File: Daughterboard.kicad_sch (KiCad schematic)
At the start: 61 parts, among them U1 SI8271GB-IS, U2 SI8271GB-IS, U3 GS61004B, U4 IES0105S09, U5 GS61004B, U6 IES0105S09

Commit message: initial version for commenting
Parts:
- TP13, TP14, TP15, TP16, TP17, TP18, TP19: footprint TestPoint:TestPoint_Pad_D2.0mm -> TestPoint:TestPoint_THTPad_D1.0mm_Drill0.5mm
- U3, U5: footprint GS61004B:GS61004B -> GS61004B:GS6XXX4B
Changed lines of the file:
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@@
 			)
 		)
-		(property "Footprint" "TestPoint:TestPoint_Pad_D2.0mm"
+		(property "Footprint" "TestPoint:TestPoint_THTPad_D1.0mm_Drill0.5mm"
 			(at 341.63 125.73 0)
 			(effects
@@
 			)
 		)
-		(property "Footprint" "TestPoint:TestPoint_Pad_D2.0mm"
+		(property "Footprint" "TestPoint:TestPoint_THTPad_D1.0mm_Drill0.5mm"
 			(at 341.503 107.823 0)
 			(effects
@@
 			)
 		)
-		(property "Footprint" "GS61004B:GS61004B"
+		(property "Footprint" "GS61004B:GS6XXX4B"
 			(at 232.41 231.14 0)
 			(effects
@@
 			)
 		)
-		(property "Footprint" "TestPoint:TestPoint_Pad_D2.0mm"
+		(property "Footprint" "TestPoint:TestPoint_THTPad_D1.0mm_Drill0.5mm"
 			(at 355.6 125.73 0)
 			(effects
@@
 			)
 		)
-		(property "Footprint" "TestPoint:TestPoint_Pad_D2.0mm"
+		(property "Footprint" "TestPoint:TestPoint_THTPad_D1.0mm_Drill0.5mm"
 			(at 325.12 125.73 0)
 			(effects
@@
 			)
 		)
-		(property "Footprint" "TestPoint:TestPoint_Pad_D2.0mm"
+		(property "Footprint" "TestPoint:TestPoint_THTPad_D1.0mm_Drill0.5mm"
 			(at 324.993 107.823 0)
 			(effects
@@
 			)
 		)
-		(property "Footprint" "TestPoint:TestPoint_Pad_D2.0mm"
+		(property "Footprint" "TestPoint:TestPoint_THTPad_D1.0mm_Drill0.5mm"
 			(at 314.96 125.73 0)
 			(effects
@@
 			)
 		)
-		(property "Footprint" "TestPoint:TestPoint_Pad_D2.0mm"
+		(property "Footprint" "TestPoint:TestPoint_THTPad_D1.0mm_Drill0.5mm"
 			(at 355.473 107.823 0)
 			(effects
@@
 			)
 		)
-		(property "Footprint" "GS61004B:GS61004B"
+		(property "Footprint" "GS61004B:GS6XXX4B"
 			(at 232.41 93.98 0)
 			(effects

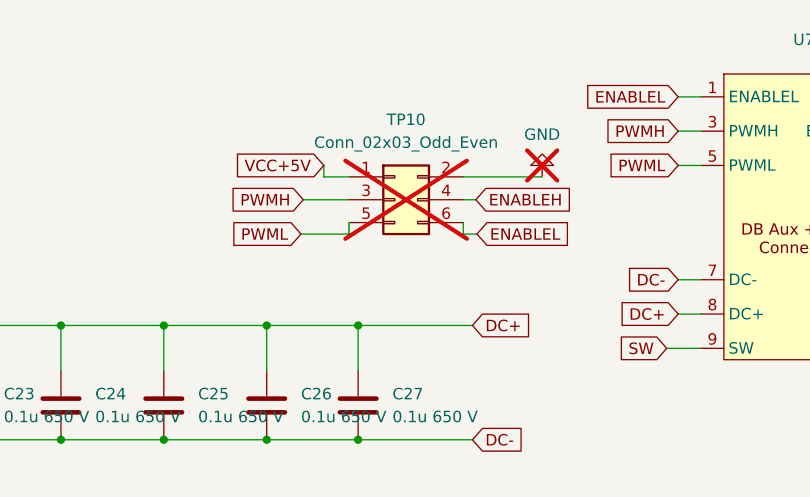
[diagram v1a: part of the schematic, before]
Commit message: fixed after comments
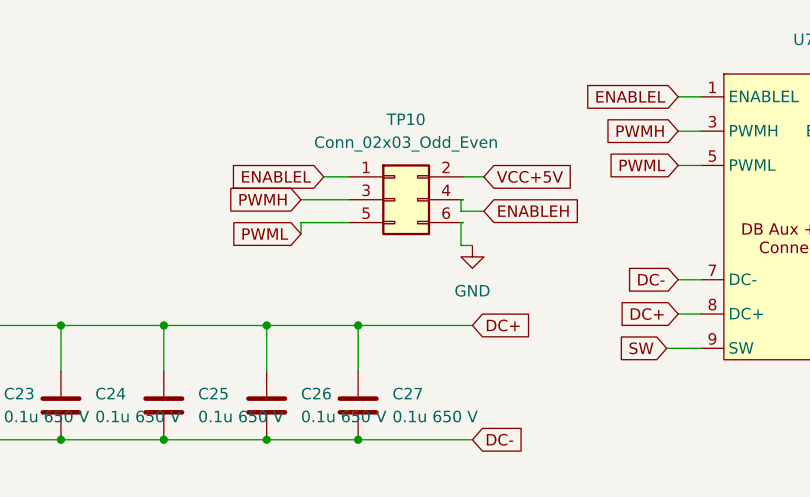
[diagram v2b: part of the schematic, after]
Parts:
- TP10: footprint (none) -> 3x2_connector:CON6_2X3_TU_TSW_SAI; now fitted
- U1, U2: footprint Package_SO:SOIC-8-1EP_3.9x4.9mm_P1.27mm_EP2.29x3mm -> Package_SO:SOIC-8_3.9x4.9mm_P1.27mm
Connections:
- net ENABLEL: now also TP10.1 (Pin_1); no longer TP10.6 (Pin_6)
- net GND: now also TP10.6 (Pin_6); no longer TP10.2 (Pin_2)
- net VCC+5V: now also TP10.2 (Pin_2); no longer TP10.1 (Pin_1)
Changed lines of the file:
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@@
 	(wire
 		(pts
-			(xy 124.46 106.68) (xy 105.41 106.68)
+			(xy 339.09 36.83) (xy 340.36 36.83)
 		)
 		(stroke
@@
 	(wire
 		(pts
-			(xy 323.85 27.94) (xy 323.85 29.21)
+			(xy 124.46 106.68) (xy 105.41 106.68)
 		)
 		(stroke
@@
 	(wire
 		(pts
+			(xy 321.31 34.29) (xy 321.31 35.56)
+		)
+		(stroke
+			(width 0)
+			(type default)
+		)
+	)
+	(wire
+		(pts
 			(xy 124.46 101.6) (xy 124.46 100.33)
 		)
@@
 	(wire
 		(pts
+			(xy 326.644 29.21) (xy 323.85 29.21)
+		)
+		(stroke
+			(width 0)
+			(type default)
+		)
+	)
+	(wire
+		(pts
 			(xy 273.05 45.72) (xy 273.05 50.8)
 		)
@@
 	(wire
 		(pts
-			(xy 339.344 35.56) (xy 339.344 34.29)
+			(xy 339.09 33.02) (xy 341.63 33.02)
 		)
 		(stroke
@@
 	(wire
 		(pts
+			(xy 339.09 34.29) (xy 339.344 34.29)
+		)
+		(stroke
+			(width 0)
+			(type default)
+		)
+	)
+	(wire
+		(pts
 			(xy 220.98 246.38) (xy 240.03 246.38)
 		)
@@
 	(wire
 		(pts
-			(xy 348.107 29.21) (xy 339.344 29.21)
-		)
-		(stroke
-			(width 0)
-			(type default)
-		)
-	)
-	(wire
-		(pts
 			(xy 176.53 24.13) (xy 176.53 26.67)
 		)
@@
 	(wire
 		(pts
+			(xy 339.09 33.02) (xy 339.09 31.75)
+		)
+		(stroke
+			(width 0)
+			(type default)
+		)
+	)
+	(wire
+		(pts
 			(xy 158.75 240.03) (xy 158.75 237.49)
 		)
@@
 	(wire
 		(pts
-			(xy 323.85 29.21) (xy 326.644 29.21)
-		)
-		(stroke
-			(width 0)
-			(type default)
-		)
-	)
-	(wire
-		(pts
 			(xy 391.16 24.13) (xy 388.62 24.13)
 		)
@@
 	(wire
 		(pts
-			(xy 326.644 35.56) (xy 326.644 34.29)
-		)
-		(stroke
-			(width 0)
-			(type default)
-		)
-	)
-	(wire
-		(pts
 			(xy 319.913 107.823) (xy 319.913 110.363)
 		)
@@
 	(wire
 		(pts
+			(xy 339.09 36.83) (xy 339.09 34.29)
+		)
+		(stroke
+			(width 0)
+			(type default)
+		)
+	)
+	(wire
+		(pts
 			(xy 190.5 185.42) (xy 179.07 185.42)
 		)
@@
 	(wire
 		(pts
-			(xy 321.564 31.75) (xy 326.644 31.75)
+			(xy 321.31 31.75) (xy 326.644 31.75)
 		)
 		(stroke
@@
 	(wire
 		(pts
+			(xy 339.09 31.75) (xy 339.344 31.75)
+		)
+		(stroke
+			(width 0)
+			(type default)
+		)
+	)
+	(wire
+		(pts
 			(xy 48.26 26.67) (xy 48.26 27.94)
 		)
@@
 	(wire
 		(pts
+			(xy 326.644 34.29) (xy 321.31 34.29)
+		)
+		(stroke
+			(width 0)
+			(type default)
+		)
+	)
+	(wire
+		(pts
 			(xy 82.55 238.76) (xy 124.46 238.76)
 		)
@@
 	(wire
 		(pts
-			(xy 340.868 35.56) (xy 339.344 35.56)
-		)
-		(stroke
-			(width 0)
-			(type default)
-		)
-	)
-	(wire
-		(pts
 			(xy 205.74 46.99) (xy 205.74 49.53)
 		)
@@
 	(wire
 		(pts
-			(xy 294.64 58.42) (xy 306.07 58.42)
+			(xy 339.344 29.21) (xy 341.63 29.21)
 		)
 		(stroke
@@
 	(wire
 		(pts
-			(xy 327.66 45.72) (xy 327.66 50.8)
+			(xy 294.64 58.42) (xy 306.07 58.42)
 		)
 		(stroke
@@
 	(wire
 		(pts
-			(xy 363.22 24.13) (xy 365.76 24.13)
+			(xy 327.66 45.72) (xy 327.66 50.8)
 		)
 		(stroke
@@
 	(wire
 		(pts
-			(xy 186.69 203.2) (xy 186.69 207.01)
+			(xy 363.22 24.13) (xy 365.76 24.13)
 		)
 		(stroke
@@
 	(wire
 		(pts
-			(xy 176.53 34.29) (xy 176.53 49.53)
+			(xy 186.69 203.2) (xy 186.69 207.01)
 		)
 		(stroke
@@
 	(wire
 		(pts
-			(xy 273.05 45.72) (xy 284.48 45.72)
+			(xy 176.53 34.29) (xy 176.53 49.53)
 		)
 		(stroke
@@
 	(wire
 		(pts
-			(xy 321.31 35.56) (xy 326.644 35.56)
+			(xy 273.05 45.72) (xy 284.48 45.72)
 		)
 		(stroke
@@
 	(wire
 		(pts
-			(xy 339.344 31.75) (xy 340.741 31.75)
-		)
-		(stroke
-			(width 0)
-			(type default)
-		)
-	)
-	(wire
-		(pts
 			(xy 82.55 101.6) (xy 124.46 101.6)
 		)
@@
 	(global_label "ENABLEH"
 		(shape input)
-		(at 340.741 31.75 0)
+		(at 341.63 33.02 0)
 		(fields_autoplaced yes)
 		(effects
@@
 		)
 		(property "Intersheetrefs" "${INTERSHEET_REFS}"
-			(at 352.0719 31.75 0)
+			(at 352.9609 33.02 0)
 			(effects
 				(font
@@
 	(global_label "PWMH"
 		(shape input)
-		(at 321.564 31.75 180)
+		(at 321.31 31.75 180)
 		(fields_autoplaced yes)
 		(effects
@@
 		)
 		(property "Intersheetrefs" "${INTERSHEET_REFS}"
-			(at 313.0755 31.75 0)
+			(at 312.8215 31.75 0)
 			(effects
 				(font
@@
 	(global_label "ENABLEL"
 		(shape input)
-		(at 340.868 35.56 0)
+		(at 323.85 29.21 180)
 		(fields_autoplaced yes)
 		(effects
@@
 				(size 1.27 1.27)
 			)
-			(justify left)
+			(justify right)
 		)
 		(property "Intersheetrefs" "${INTERSHEET_REFS}"
-			(at 351.8965 35.56 0)
+			(at 312.8215 29.21 0)
 			(effects
 				(font
 					(size 1.27 1.27)
 				)
-				(justify left)
+				(justify right)
 				(hide yes)
 			)
@@
 	(global_label "VCC+5V"
 		(shape input)
-		(at 323.85 27.94 180)
+		(at 341.63 29.21 0)
 		(fields_autoplaced yes)
 		(effects
@@
 				(size 1.27 1.27)
 			)
-			(justify right)
+			(justify left)
 		)
 		(property "Intersheetrefs" "${INTERSHEET_REFS}"
-			(at 313.3657 27.94 0)
+			(at 352.1143 29.21 0)
 			(effects
 				(font
 					(size 1.27 1.27)
 				)
-				(justify right)
+				(justify left)
 				(hide yes)
 			)
@@
 	(symbol
 		(lib_id "power:GND")
-		(at 348.107 29.21 180)
+		(at 340.36 36.83 0)
 		(unit 1)
 		(exclude_from_sim no)
 		(in_bom yes)
 		(on_board yes)
-		(dnp yes)
+		(dnp no)
 		(fields_autoplaced yes)
 		(property "Reference" "#PWR014"
-			(at 348.107 22.86 0)
+			(at 340.36 43.18 0)
 			(effects
 				(font
@@
 		)
 		(property "Value" "GND"
-			(at 348.107 24.511 0)
+			(at 340.36 41.91 0)
 			(effects
 				(font
@@
 		)
 		(property "Footprint" ""
-			(at 348.107 29.21 0)
+			(at 340.36 36.83 0)
 			(effects
 				(font
@@
 		)
 		(property "Datasheet" ""
-			(at 348.107 29.21 0)
+			(at 340.36 36.83 0)
 			(effects
 				(font
@@
 		)
 		(property "Description" ""
-			(at 348.107 29.21 0)
+			(at 340.36 36.83 0)
 			(effects
 				(font
@@
 			)
 		)
-		(property "Footprint" "Package_SO:SOIC-8-1EP_3.9x4.9mm_P1.27mm_EP2.29x3mm"
+		(property "Footprint" "Package_SO:SOIC-8_3.9x4.9mm_P1.27mm"
 			(at 149.86 242.57 0)
 			(effects
@@
 		(in_bom yes)
 		(on_board yes)
-		(dnp yes)
+		(dnp no)
 		(fields_autoplaced yes)
 		(property "Reference" "TP10"
@@
 			)
 		)
-		(property "Footprint" ""
+		(property "Footprint" "3x2_connector:CON6_2X3_TU_TSW_SAI"
 			(at 331.724 31.75 0)
 			(effects
@@
 			)
 		)
-		(property "Footprint" "Package_SO:SOIC-8-1EP_3.9x4.9mm_P1.27mm_EP2.29x3mm"
+		(property "Footprint" "Package_SO:SOIC-8_3.9x4.9mm_P1.27mm"
 			(at 149.86 105.41 0)
 			(effects
